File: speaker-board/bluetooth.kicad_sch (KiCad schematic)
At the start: 0 parts

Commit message: updates
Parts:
- added U3: Microchip_BM83, RF_Module:Microchip_BM83, symbol RF_Bluetooth:Microchip_BM83
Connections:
- new net +3.3V: U3.23 (BAT_IN)
- new net GND: U3.16 (GND), U3.50 (GND), U3.56 (GND), U3.57 (GND)
- new net UART_RX: U3.29 (P8_6/UART_RXD)
- new net UART_TX: U3.30 (P8_5/UART_TXD)

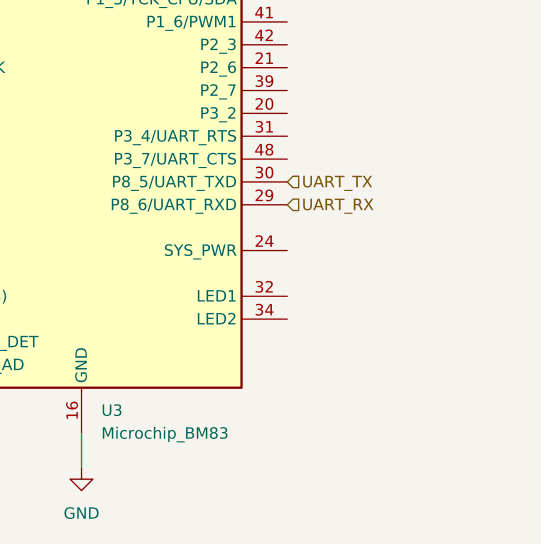
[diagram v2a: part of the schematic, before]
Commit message: update
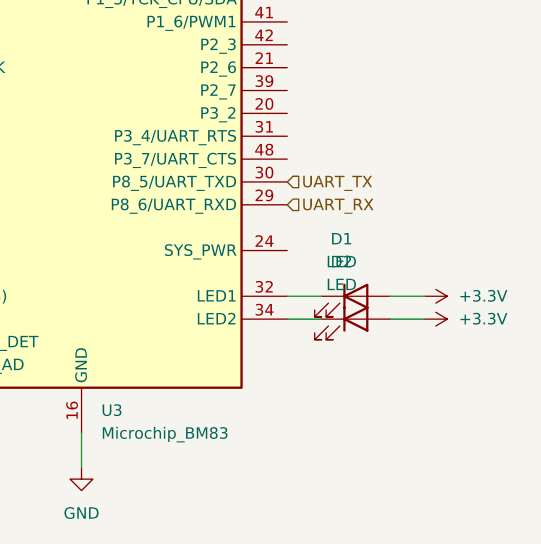
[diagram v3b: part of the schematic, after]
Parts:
- added D1, D2: LED, symbol Device:LED
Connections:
- net +3.3V: now also D1.2 (A), D2.2 (A)
- net at U3.32 (LED1): now also D1.1 (K)
- net at U3.34 (LED2): now also D2.1 (K)
